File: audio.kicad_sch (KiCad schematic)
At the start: 38 parts, among them IC1 TAC5212IRGER, J16 Debug, J18 Jack 6.35mm, J19 Jack 6.35mm, J20 Jack 6.35mm, J22 Jack 6.35mm, U14 OPA1656ID, U7 74AHCT1G32SE-7

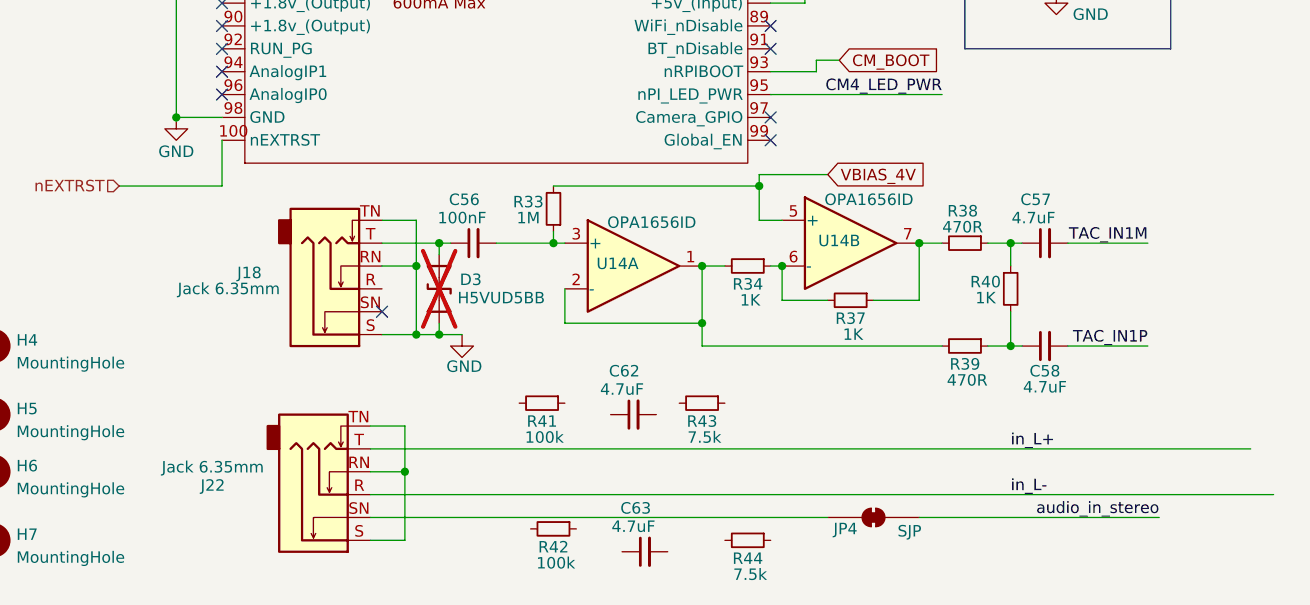
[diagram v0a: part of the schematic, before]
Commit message: updated docs from chatgpt discussions.
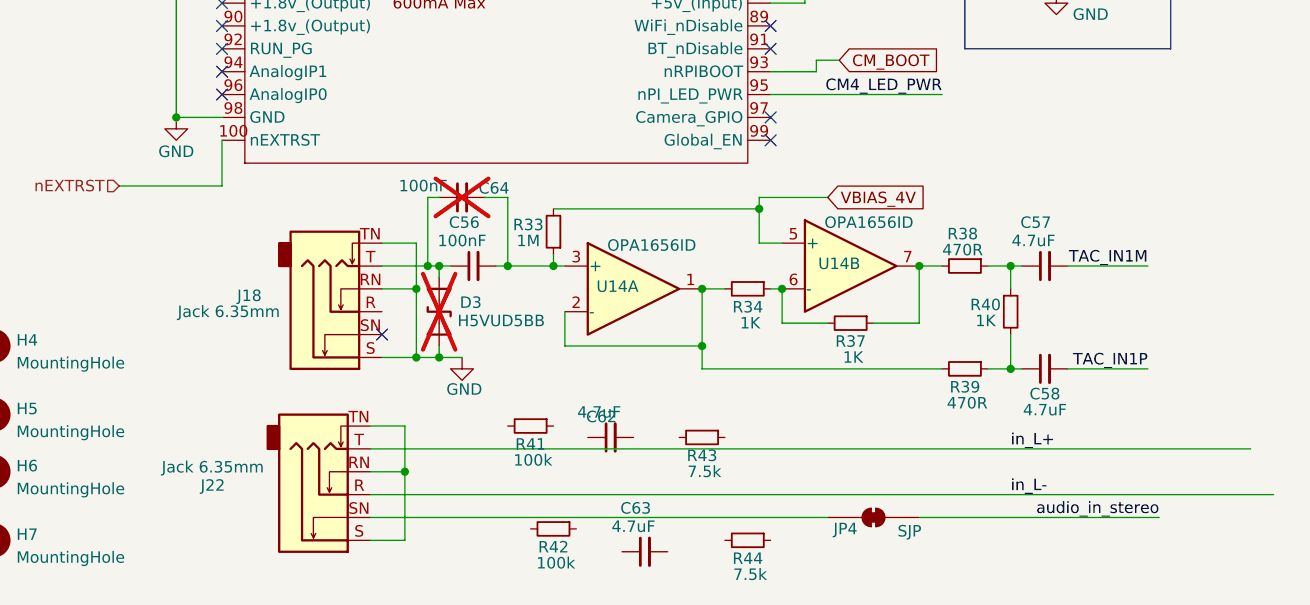
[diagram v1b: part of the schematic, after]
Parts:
- added C64: 100nF, Capacitor_SMD:C_1206_3216Metric_Pad1.33x1.80mm_HandSolder, symbol Device:C_Small
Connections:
- net at C56.2, R33.1, U14.3 (+): now also C64.2
- net at C56.1, D3.2 (A2), J18.T: now also C64.1
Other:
- moved on the sheet: C56, C57, C58, C62, D3, J18, R33, R34, R37, R38, R39, R40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
